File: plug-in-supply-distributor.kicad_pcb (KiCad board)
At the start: 2 copper layers, 60 x 30 mm, 37 parts, among them J1 Conn_02x18_Odd_Even, J2 Conn_02x04_Odd_Even, J3 PV-3, J4 PV-3, J5 PV-3, Q1 2N7002K, Q2 SUD50P04-08, Q3 2N7002K, Q4 SUD50P04-08, U1 74LS27, U2 BD450M5FP

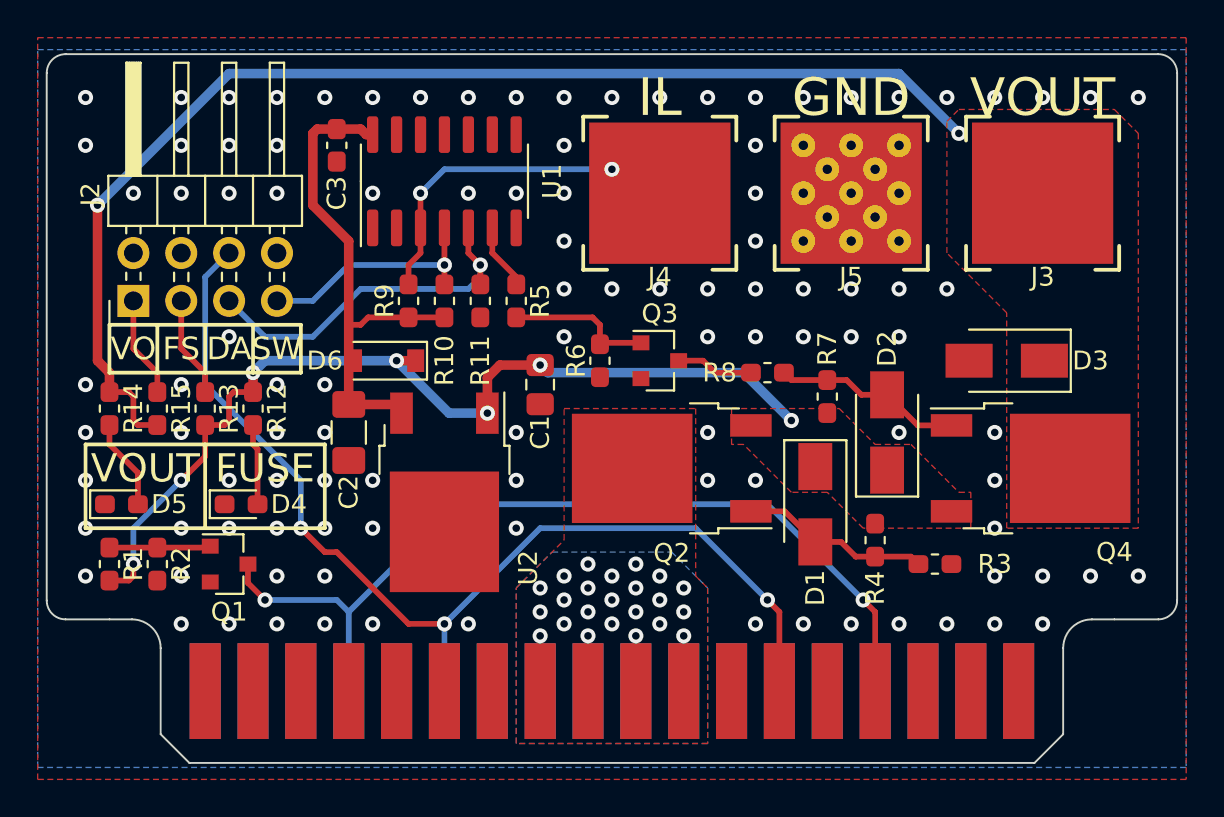
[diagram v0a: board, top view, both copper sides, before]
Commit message: Update kicad files
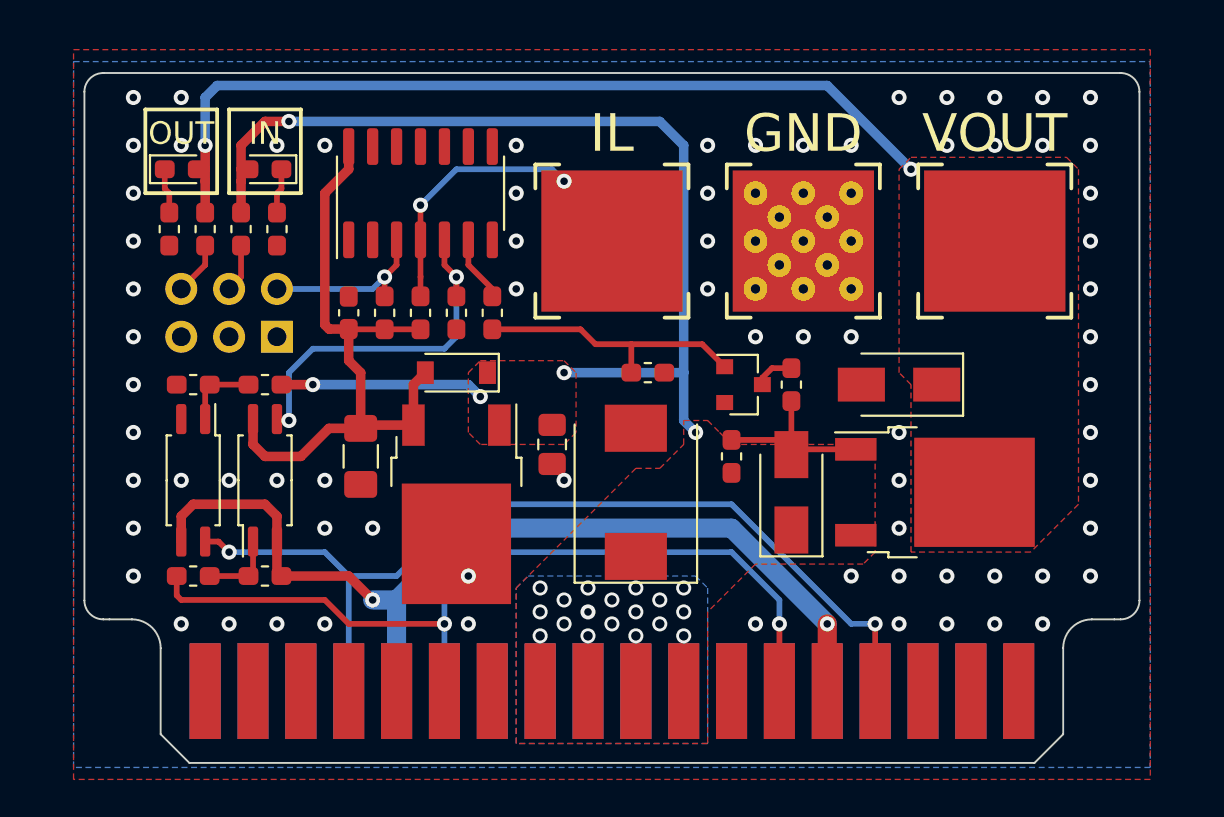
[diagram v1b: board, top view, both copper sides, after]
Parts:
- removed the D2 at (114.6, 105.1)
- removed Q3: 2N7002K, Package_TO_SOT_SMD:SOT-23
- removed Q4: SUD50P04-08, Package_TO_SOT_SMD:TO-252-2
- removed the R3 at (117.1, 112.1)
- removed the R7 at (111.4, 103.2)
- removed the R8 at (108.3, 101.9)
- removed the REF** at (124.8, 103.8)
- added D6: B340A-13-F, Diode_SMD:D_SMA, F.Cu at (115.2, 102.5)
- added R11: 10k, Resistor_SMD:R_0603_1608Metric_Pad1.05x0.95mm_HandSolder, F.Cu at (106.3, 106.3)
- added R12: 20k, Resistor_SMD:R_0603_1608Metric_Pad1.05x0.95mm_HandSolder, F.Cu at (109.5, 102.5)
- added R5: 4.7k, Resistor_SMD:R_0603_1608Metric_Pad1.05x0.95mm_HandSolder, F.Cu at (81.6, 102.5)
- added U1: TLP291, Package_SO:SOIC-4_4.55x2.6mm_P1.27mm, F.Cu at (81.6, 107.6)
- added U2: TLP291, Package_SO:SOIC-4_4.55x2.6mm_P1.27mm, F.Cu at (77.8, 107.6)
- D1: value SMAJ12CA-E3/61 -> D_Zener; footprint Diode_SMD:D_SMA -> Diode_SMD:D_SMC
- D3: value B340A-13-F -> SMAJ12CA-E3/61
- D4: renamed from D6; value B340A-13-F -> RB162M-40TR
- J2: value Conn_02x04_Odd_Even -> Conn_02x03_Odd_Even; footprint Connector_PinHeader_2.54mm:PinHeader_2x04_P2.54mm_Horizontal -> Connector_PinHeader_2.54mm:PinHeader_2x03_P2.54mm_Horizontal; moved to B.Cu
- R1: value 20k -> 4.7k
- R2, R4: value 10k -> 1k
- moved R4 37.1 mm to (77.8, 102.5), turned to 180 degrees
- moved Q1 28.9 mm to (107.0, 102.5)
- moved D5 18.1 mm to (77.1, 91.1)
- moved D2 17.8 mm to (81.6, 91.1), turned to 180 degrees
- moved Q2 14.0 mm to (117.1, 108.3), turned to 0 degrees
- moved D3 13.4 mm to (109.5, 108.3), turned to 90 degrees
- moved R13 10.0 mm to (76.5, 94.3)
- moved R15 9.86 mm to (78.4, 94.3), turned to 270 degrees
- moved R14 9.71 mm to (80.3, 94.3), turned to 270 degrees
- moved R9 9.61 mm to (82.2, 94.3)
- moved D1 9.55 mm to (101.3, 108.3), turned to 90 degrees
- moved C3 8.91 mm to (86.0, 98.7), turned to 90 degrees
- moved J2 7.85 mm to (82.2, 100.0)
- moved R2 5.75 mm to (81.6, 112.7), turned to 0 degrees
- moved R1 4.49 mm to (77.8, 112.7), turned to 180 degrees
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- renumbered D4 to D2, R6 to R10, R14 to R13, R13 to R14, R11 to R3, R10 to R6, R9 to R7, R5 to R8, R12 to R9, U1 to U3, U2 to U4
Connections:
- C1 pad 1: /vp -> /vin
- C1 pad 2: GND -> GNDPWR
- C2 pad 2: GND -> GNDPWR
- C3 pad 2: GND -> GNDPWR
- D1 pad 1: /vp -> /vin
- D1 pad 2: Net-(D1-Pad2) -> GNDPWR
- D2 pad 1: GND -> Net-(D2-Pad1)
- D2 pad 2: Net-(D4-Pad2) -> /vin
- D3 pad 1: /vout -> /vin
- D3 pad 2: GND -> Net-(D3-Pad2)
- D4 pad 1: /vp -> /vin
- D5 pad 1: GND -> Net-(D5-Pad1)
- D5 pad 2: Net-(D5-Pad2) -> /vout
- J1 pad 1: GND -> GNDPWR
- J1 pad 11: GND -> GNDPWR
- J1 pad 13: GND -> GNDPWR
- J1 pad 14: GND -> GNDPWR
- J1 pad 2: GND -> GNDPWR
- J1 pad 23: GND -> GNDPWR
- J1 pad 24: GND -> GNDPWR
- J1 pad 26: GND -> GNDPWR
- J1 pad 28: GND -> GNDPWR
- J1 pad 3: GND -> GNDPWR
- J1 pad 30: GND -> GNDPWR
- J1 pad 31: GND -> GNDPWR
- J1 pad 32: GND -> GNDPWR
- J1 pad 33: GND -> GNDPWR
- J1 pad 34: GND -> GNDPWR
- J1 pad 35: GND -> GNDPWR
- J1 pad 36: GND -> GNDPWR
- J1 pad 4: GND -> GNDPWR
- J1 pad 5: GND -> GNDPWR
- J1 pad 6: GND -> GNDPWR
- J1 pad 7: GND -> GNDPWR
- J1 pad 9: GND -> GNDPWR
- J2 pad 1: Net-(J2-Pad1) -> GNDPWR
- J2 pad 2: GND -> /sw
- J2 pad 3: Net-(J2-Pad3) -> GNDPWR
- J2 pad 4: GND -> Net-(J2-Pad4)
- J2 pad 5: Net-(J2-Pad5) -> GNDPWR
- J2 pad 6: /disable -> Net-(J2-Pad6)
- J5 pad 1: GND -> GNDPWR
- Q1 pad 2: GND -> GNDPWR
- Q1 pad 3: /fuse_status_out_od -> Net-(Q1-Pad3)
- Q2 pad 1: Net-(D1-Pad2) -> Net-(D3-Pad2)
- Q2 pad 2: /vin -> /vout
- Q2 pad 3: /vp -> /vin
- R1 pad 1: Net-(Q1-Pad1) -> Net-(R1-Pad1)
- R1 pad 2: /vp -> /disable
- R10 pad 1: Net-(Q3-Pad1) -> Net-(Q1-Pad1)
- R10 pad 2: GND -> GNDPWR
- R13 pad 1: /vout -> Net-(D5-Pad1)
- R13 pad 2: Net-(D5-Pad2) -> GNDPWR
- R14 pad 1: /vp -> /vin
- R14 pad 2: Net-(J2-Pad3) -> Net-(J2-Pad4)
- R15 pad 2: Net-(J2-Pad1) -> Net-(J2-Pad6)
- R2 pad 1: Net-(Q1-Pad1) -> Net-(R1-Pad1)
- R3 pad 1: Net-(J2-Pad5) -> Net-(R3-Pad1)
- R3 pad 2: GND -> GNDPWR
- R4 pad 1: /vp -> Net-(R4-Pad1)
- R4 pad 2: Net-(D1-Pad2) -> GNDPWR
- R6 pad 2: /sw_in -> /interlock
- R7 pad 2: /interlock -> /sw
- R8 pad 1: Net-(Q3-Pad1) -> Net-(Q1-Pad1)
- R9 pad 1: /vp -> Net-(D2-Pad1)
- R9 pad 2: Net-(D4-Pad2) -> GNDPWR
- U3 pad 1: GND -> GNDPWR
- U3 pad 10: GND -> GNDPWR
- U3 pad 11: GND -> GNDPWR
- U3 pad 13: GND -> GNDPWR
- U3 pad 2: GND -> GNDPWR
- U3 pad 3: /interlock -> /sw
- U3 pad 4: /sw_in -> /interlock
- U3 pad 5: Net-(J2-Pad5) -> Net-(R3-Pad1)
- U3 pad 7: GND -> GNDPWR
- U3 pad 9: GND -> GNDPWR
- U4 pad 1: /vp -> /vin
- U4 pad 2: GND -> GNDPWR
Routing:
- net /vin: track 0.00 -> 61.2 mm
- net GND: track 0.00 -> 51.8 mm, vias 107 -> 2
- net /vp: track 50.4 -> 0.00 mm, vias 7 -> 0
- net Net-(J2-Pad5): track 19.3 -> 0.00 mm, vias 1 -> 0
- net Net-(R3-Pad1): track 0.00 -> 19.3 mm, vias 0 -> 2
- net /vout: track 64.1 -> 46.1 mm
- net /sw_in: track 12.7 -> 0.00 mm, vias 1 -> 0
- net /disable: track 56.5 -> 46.2 mm, vias 3 -> 2
- net Net-(D2-Pad2): track 10.1 -> 0.00 mm
- net Net-(D1-Pad2): track 10.1 -> 0.00 mm
- net Net-(D3-Pad2): track 0.00 -> 9.87 mm
- net Net-(Q1-Pad1): track 5.38 -> 14.7 mm
- net /sw: track 0.00 -> 9.24 mm, vias 0 -> 1
- net Net-(Q3-Pad1): track 7.84 -> 0.00 mm
- net VDD: track 27.1 -> 34.7 mm
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- added copper zone on B.Cu, net GNDPWR
- added copper zone on F.Cu, net GNDPWR
- removed copper zone on F.Cu, net /vp
- removed copper zone on B.Cu, net GND
- removed copper zone on F.Cu, net GND
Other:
- board size 60 x 30 mm -> 56 x 29 mm
- board text added: "FUSE LED"
- board text added: "IN"
- board text added: "OUT"
- board text added: "SWITCH"
- board text added: "VOUT LED"
- board text removed: "DA"
- board text removed: "FS"
- board text removed: "FUSE"
- board text removed: "SW"
- board text removed: "VO"
- board text removed: "VOUT"
